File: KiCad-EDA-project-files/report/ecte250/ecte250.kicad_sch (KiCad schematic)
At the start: 13 parts, among them SW1 SW_SPST, SW2 SW_SPST, SW3 SW_SPST, SW4 SW_SPST, SW5 SW_SPST, U1 LM2596S-5, U2 ADXL343

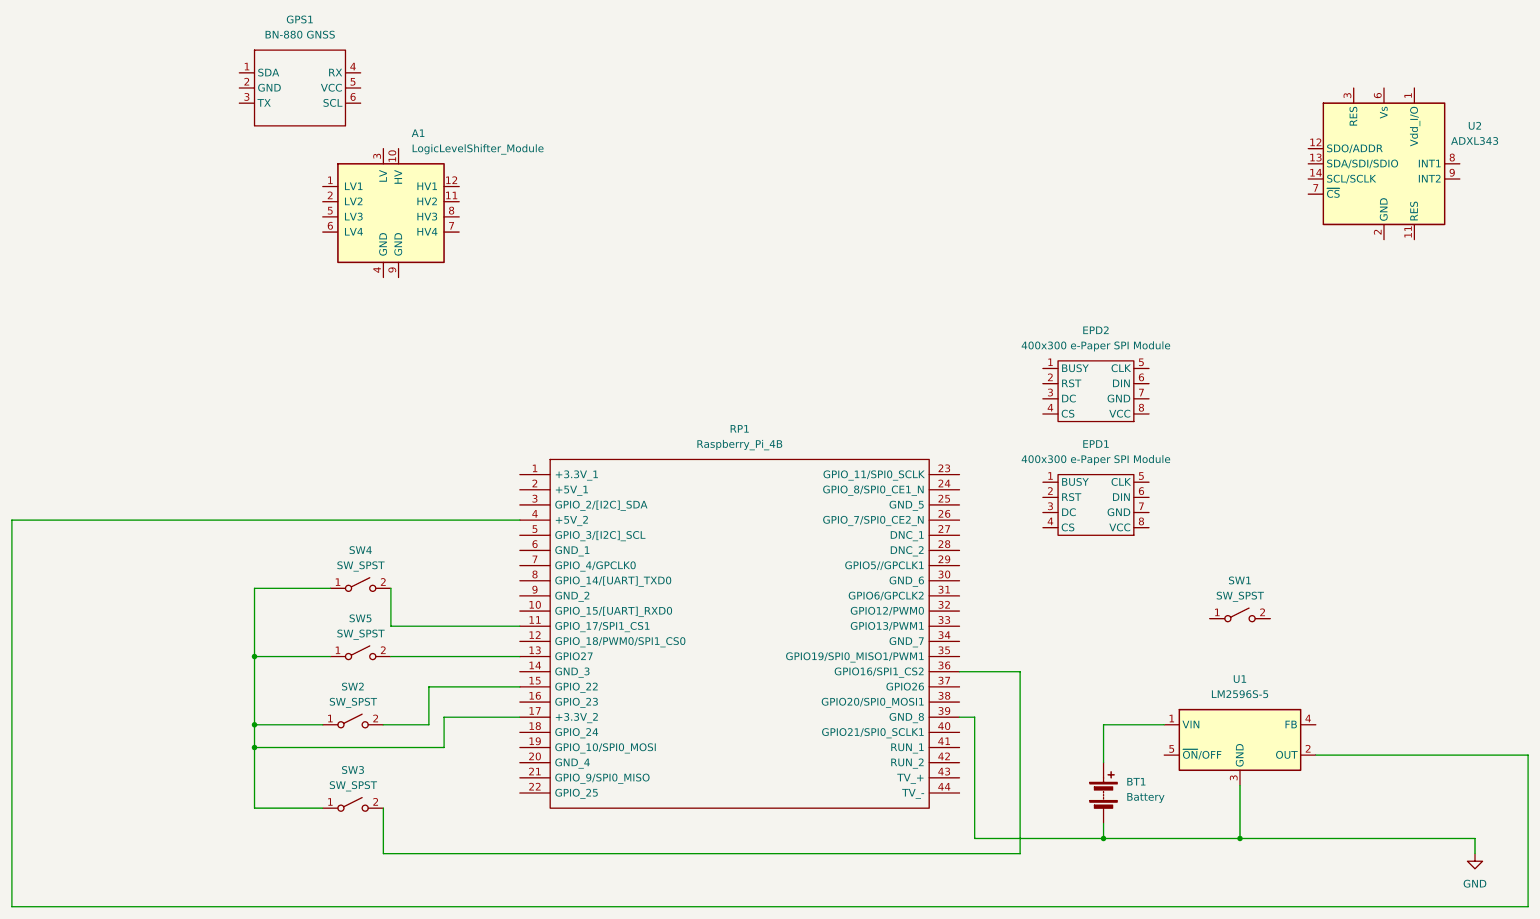
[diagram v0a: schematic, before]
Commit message: updated schematic files
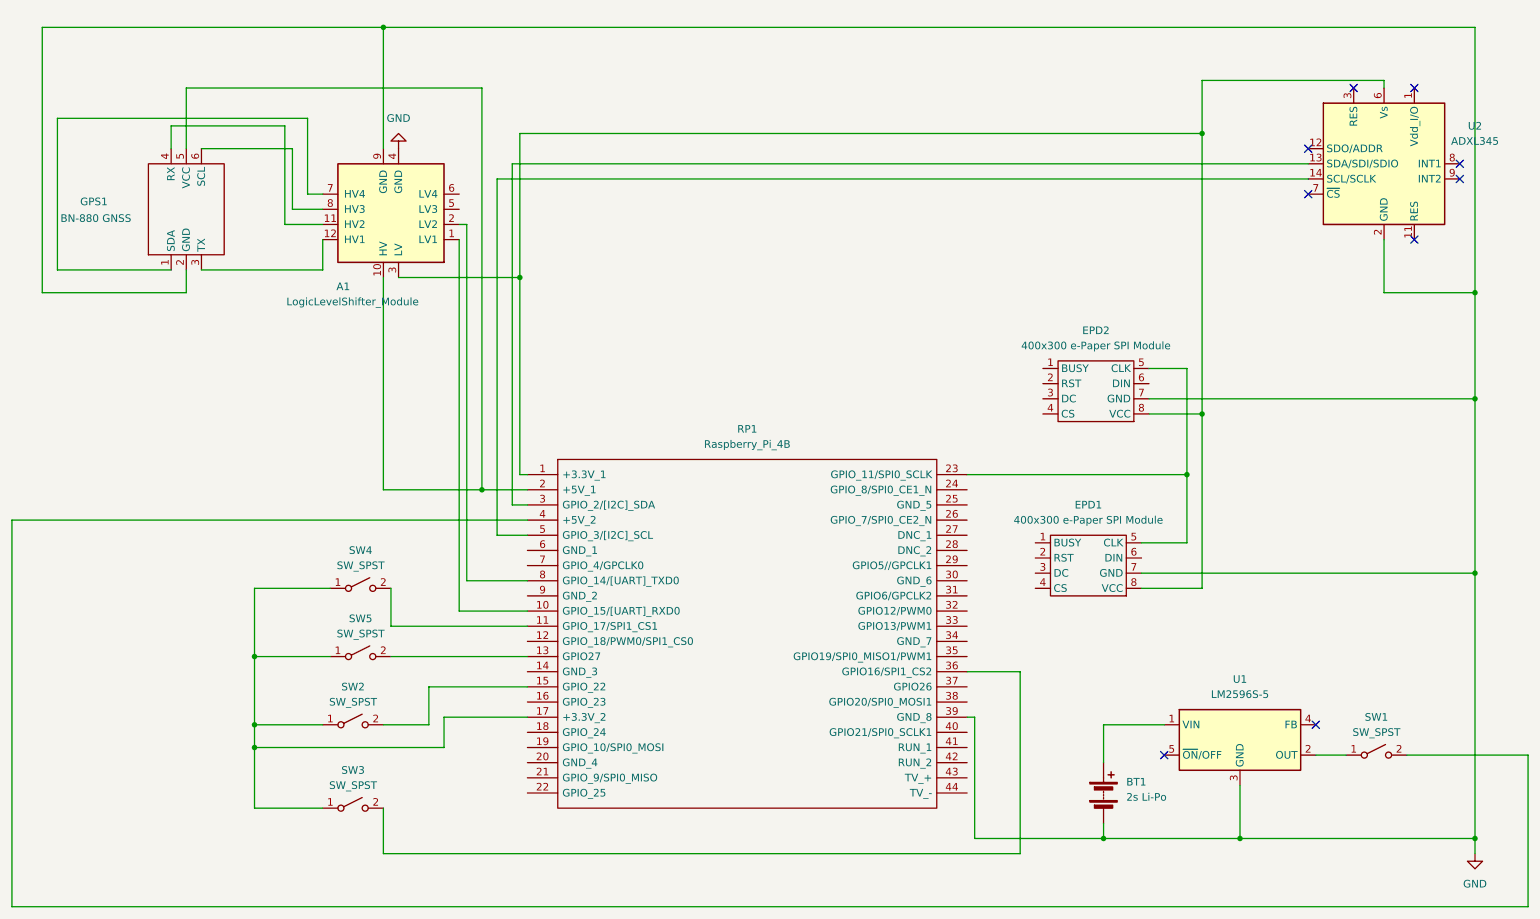
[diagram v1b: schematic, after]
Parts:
- BT1: value Battery -> 2s Li-Po
- U2: value ADXL343 -> ADXL345
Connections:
- net GND: now also A1.4 (GND), A1.9 (GND), EPD1.7 (GND), EPD2.7 (GND), GPS1.2 (GND), U2.2 (GND), U2.4 (GND), U2.5 (GND)
- net at U1.2 (OUT): now also SW1.1 (A); no longer RP1.4 (+5V_2)
- net at A1.1 (LV1): now also RP1.10 (GPIO_15/[UART]_RXD0)
- net at A1.10 (HV): now also GPS1.5 (VCC), RP1.2 (+5V_1)
- net at A1.11 (HV2): now also GPS1.4 (RX)
- net at A1.12 (HV1): now also GPS1.3 (TX)
- net at A1.2 (LV2): now also RP1.8 (GPIO_14/[UART]_TXD0)
- net at A1.3 (LV): now also EPD1.8 (VCC), EPD2.8 (VCC), RP1.1 (+3.3V_1), U2.6 (Vs)
- net at A1.7 (HV4): now also GPS1.1 (SDA)
- net at A1.8 (HV3): now also GPS1.6 (SCL)
- net at SW1.2 (B): now also RP1.4 (+5V_2)
- net at RP1.23 (GPIO_11/SPI0_SCLK): now also EPD1.5 (CLK), EPD2.5 (CLK)
- net at RP1.3 (GPIO_2/[I2C]_SDA): now also U2.13 (SDA/SDI/SDIO)
- net at RP1.5 (GPIO_3/[I2C]_SCL): now also U2.14 (SCL/SCLK)
- no-connect marks 0 -> 9
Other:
- moved on the sheet: A1, EPD1, GPS1, RP1, SW1
